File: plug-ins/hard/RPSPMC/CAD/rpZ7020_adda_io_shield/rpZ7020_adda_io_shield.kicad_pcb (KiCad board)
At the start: 4 copper layers, 61.3 x 89.9 mm, 26 parts, among them J1 Samtec_ASP-134486-01, J2-FMC-RP1 Conn_02x20, J3-FMC-POWER1 Conn_02x06_Odd_Even, J4-FMC-AUX1 Conn_02x06_Odd_Even

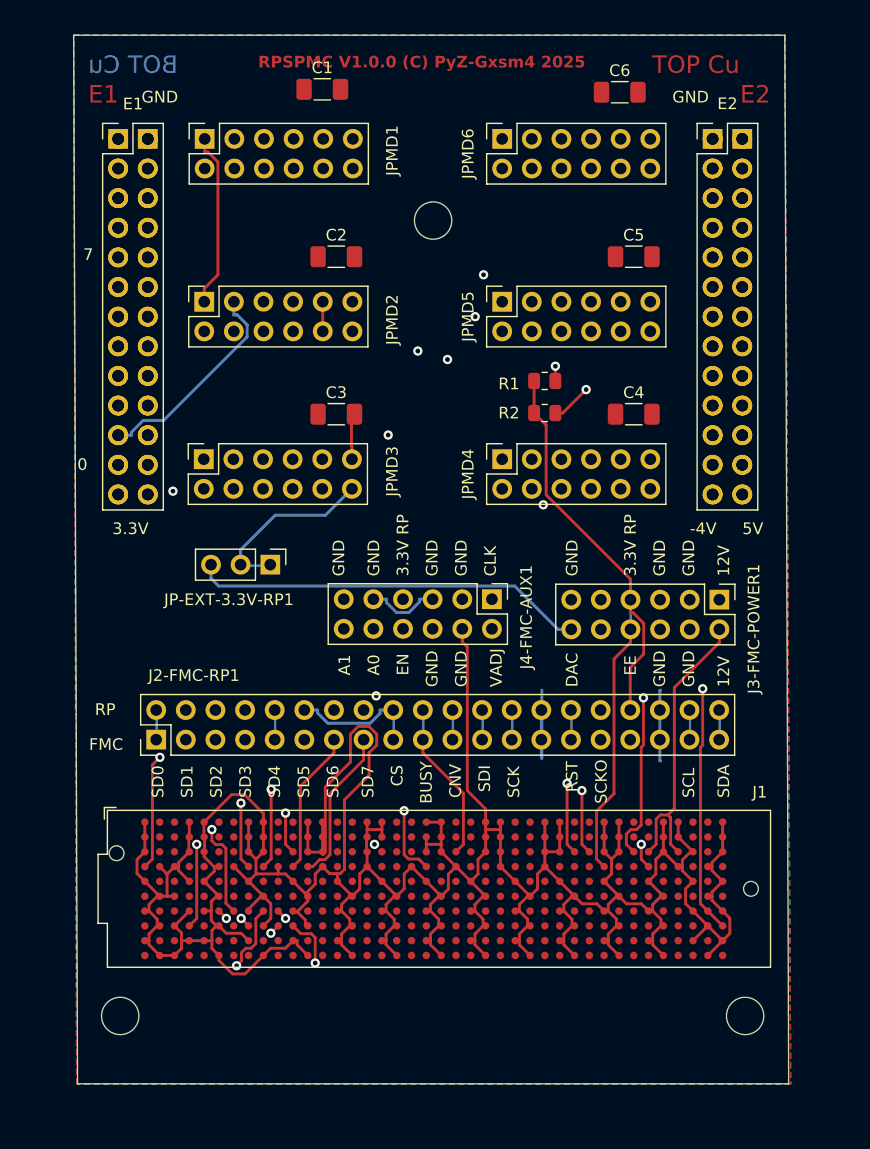
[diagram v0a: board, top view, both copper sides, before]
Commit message: work ok hat
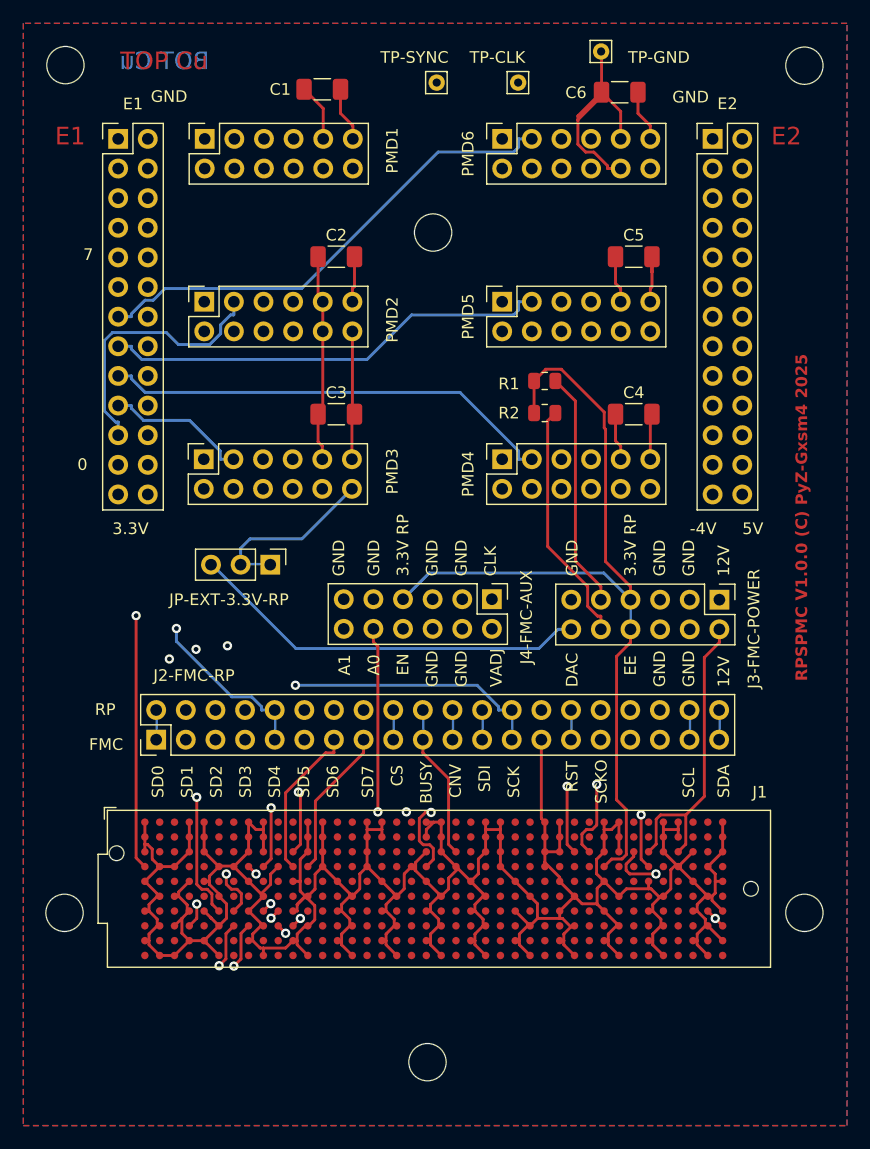
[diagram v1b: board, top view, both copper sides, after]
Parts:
- removed the E1 at (124.5, 83.8)
- removed the E1 at (175.4, 83.8)
- removed MH0: MountingHole_3.2mm_M3, MountingHole:MountingHole_3.2mm_M3
- added MH2: MountingHole_3.2mm_M3, MountingHole:MountingHole_3.2mm_M3, F.Cu at (148.4, 163.0)
- added MH3: MountingHole_3.2mm_M3, MountingHole:MountingHole_3.2mm_M3, F.Cu at (180.7, 150.2)
- added MH4: MountingHole_3.2mm_M3, MountingHole:MountingHole_3.2mm_M3, F.Cu at (180.7, 77.6)
- added MH6: MountingHole_3.2mm_M3, MountingHole:MountingHole_3.2mm_M3, F.Cu at (117.4, 77.5)
- added TP-CLK: TestPoint, Connector_Pin:Pin_D0.7mm_L6.5mm_W1.8mm_FlatFork, F.Cu at (156.2, 79.0)
- added TP-GND: TestPoint, Connector_Pin:Pin_D0.7mm_L6.5mm_W1.8mm_FlatFork, F.Cu at (163.3, 76.3)
- added TP-SYNC: TestPoint, Connector_Pin:Pin_D0.7mm_L6.5mm_W1.8mm_FlatFork, F.Cu at (149.2, 79.0)
- moved MH1 59.0 mm to (117.3, 150.2)
- moved MH5 1.03 mm to (148.9, 91.9)
- renumbered J2-FMC-RP1 to J2-FMC-RP, J3-FMC-POWER1 to J3-FMC-POWER, J4-FMC-AUX1 to J4-FMC-AUX, JP-EXT-3.3V-RP1 to JP-EXT-3.3V-RP, MH3 to MH5, JPMD1 to PMD1, JPMD2 to PMD2, JPMD3 to PMD3, JPMD4 to PMD4, JPMD5 to PMD5, JPMD6 to PMD6
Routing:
- net D2P RP: track 86.4 -> 62.0 mm, vias 2 -> 0
- net +3.3V: track 108.0 -> 127.5 mm
- net CLK-ADC: track 44.1 -> 61.1 mm
- net SYNC PMOD: track 93.9 -> 109.5 mm
- net D5P RP: track 65.6 -> 54.7 mm
- net SDO2 FMC: track 26.9 -> 16.9 mm
- net EN: track 36.3 -> 45.2 mm
- net D3P RP: track 55.3 -> 46.4 mm, vias 1 -> 0
- net CNV FMC: track 26.2 -> 34.9 mm
- net SCLK PMOD: track 104.8 -> 113.2 mm
- net SCK FMC: track 31.9 -> 40.2 mm
- net SDO5 FMC: track 24.0 -> 17.1 mm
- net SDO1 FMC: track 18.2 -> 25.1 mm
- net SDO0 FMC: track 19.3 -> 25.6 mm, vias 0 -> 1
- net VADJ: track 41.4 -> 35.3 mm
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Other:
- board outline removed
